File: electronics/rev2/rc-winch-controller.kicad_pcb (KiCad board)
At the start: 2 copper layers, 30 x 16 mm, 13 parts, among them J1 Conn_01x06, J2 Conn_01x06, SW1 SETUP, U1 MCP1703A-3302_SOT23, U2 LPC812M001JDH16, U3 RZ7889

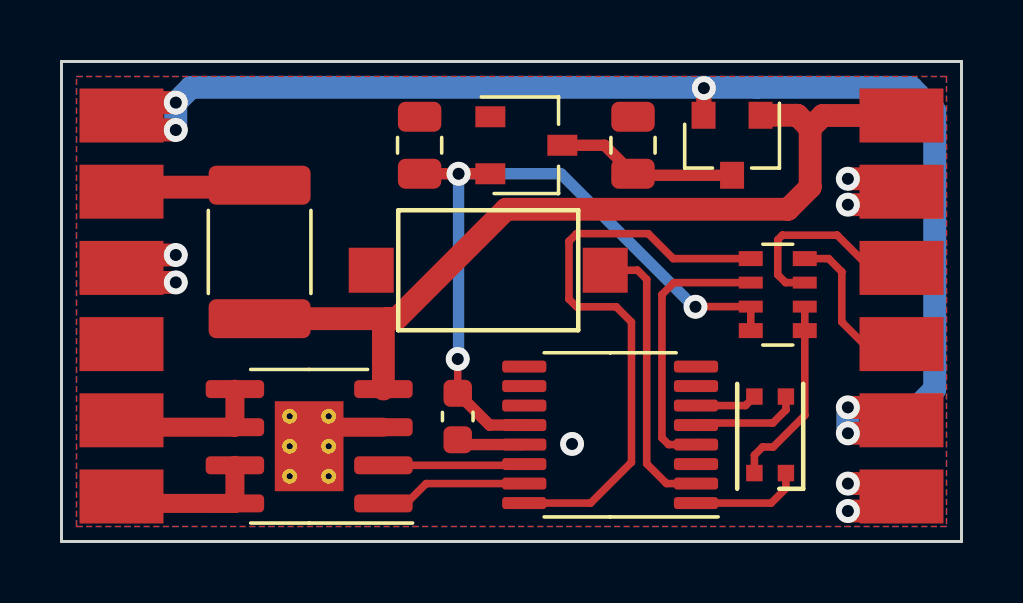
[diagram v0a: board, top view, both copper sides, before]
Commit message: Tweak placement, layout and silk screen
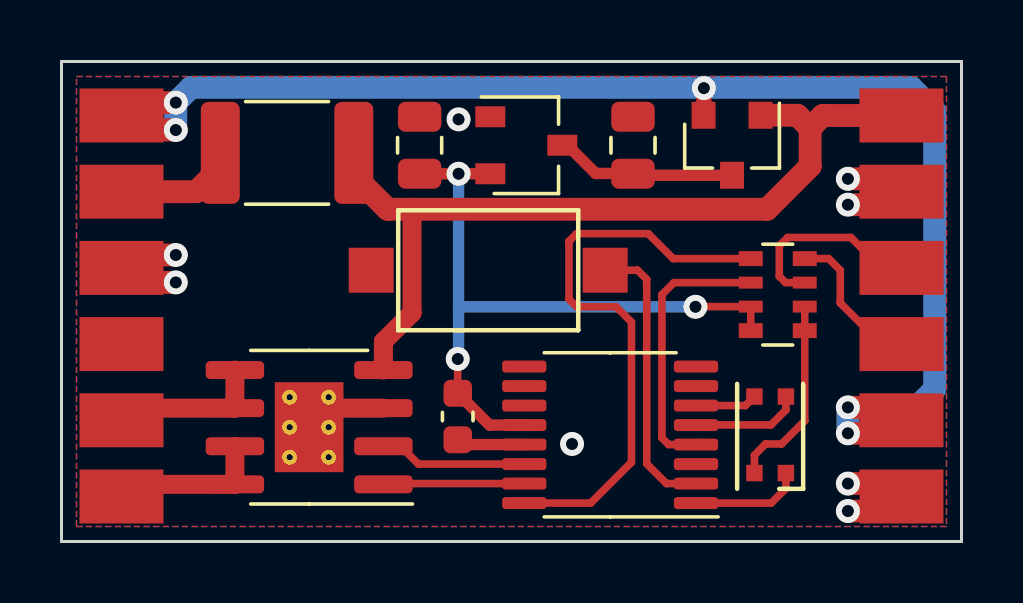
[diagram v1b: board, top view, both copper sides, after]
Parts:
- moved F1 3.43 mm to (107.5, 87.0), turned to 0 degrees
- moved U3 0.64 mm to (108.3, 96.2)
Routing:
- net /VDD: track 24.7 -> 22.9 mm
- net GND: track 16.9 -> 17.8 mm, vias 7 -> 8
- net /VMOT-in: track 4.69 -> 4.12 mm
